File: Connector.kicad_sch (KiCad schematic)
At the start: 6 parts, among them J1 UJ20-C-H-G-SMT-1-P16-TR, J2 Conn_01x02_Socket, J3 DF40C, J4 DF40C

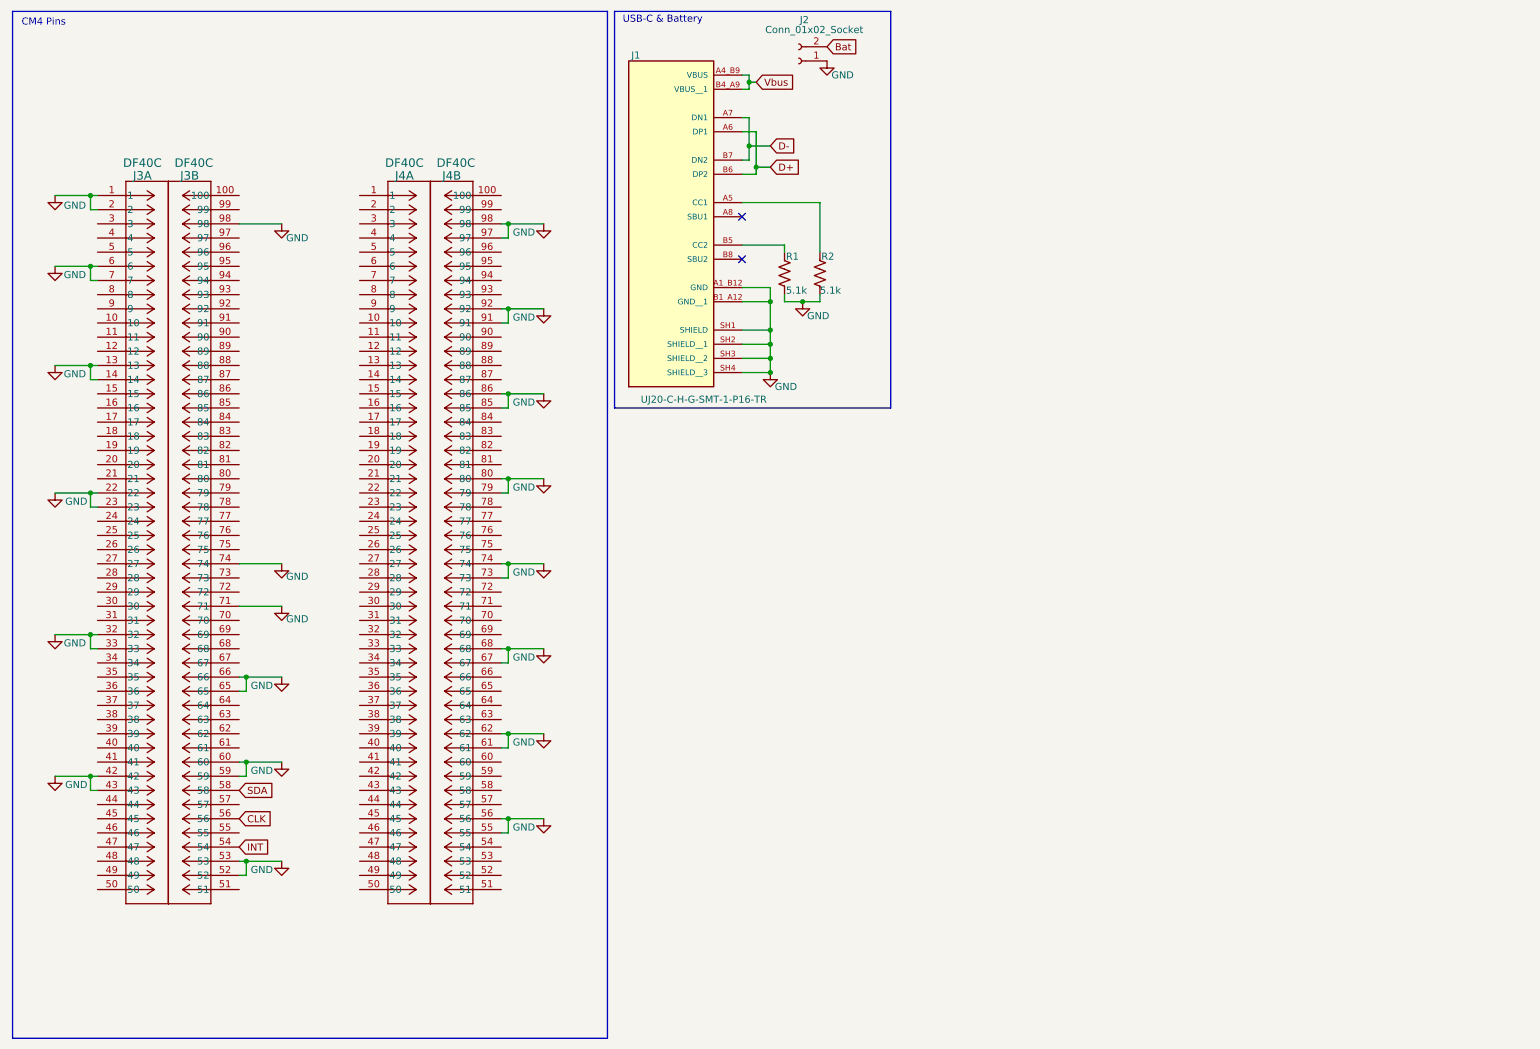
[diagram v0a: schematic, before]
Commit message: Final Schematic
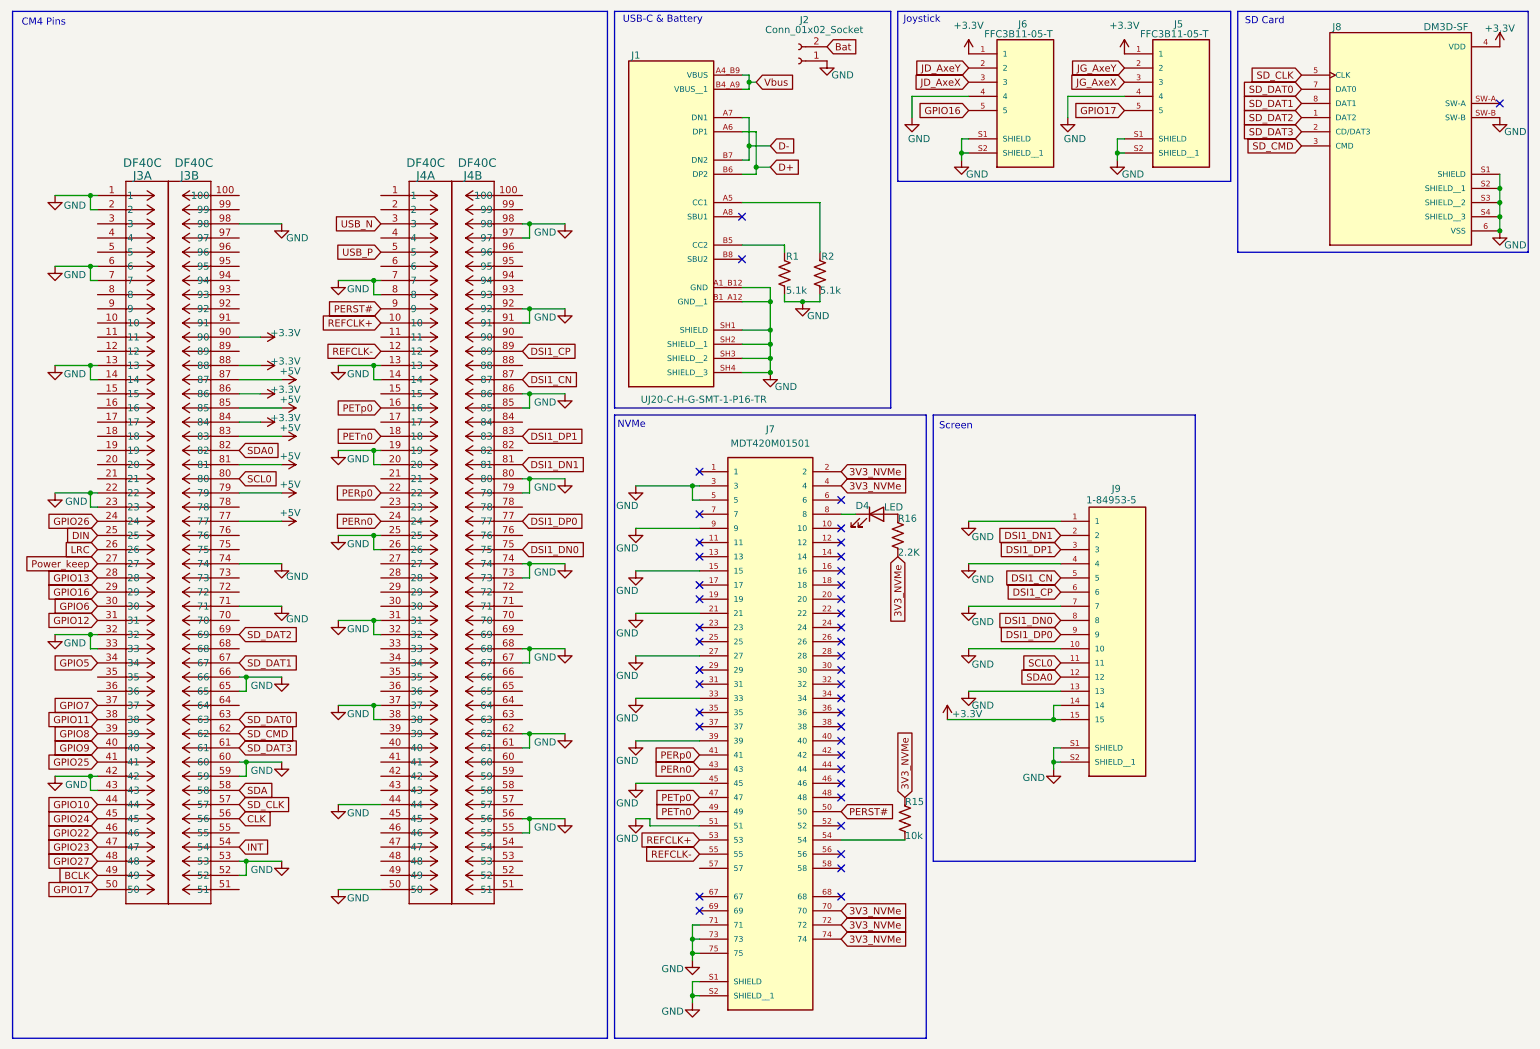
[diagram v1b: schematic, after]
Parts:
- added D4: LED, symbol Device:LED
- added J5, J6: FFC3B11-05-T, FFC3B11-05-T:GCT_FFC3B11-05-T, symbol FFC3B11-05-T:FFC3B11-05-T
- added J7: MDT420M01501, MDT420M01501:AMPHENOL_MDT420M01501, symbol MDT420M01501:MDT420M01501
- added J8: DM3D-SF, DM3D-SF:HRS_DM3D-SF, symbol DM3D-SF:DM3D-SF
- added J9: 1-84953-5, 1-84953-5:TE_1-84953-5, symbol Conn_FPC_15p:1-84953-5
- added R15: 10k, symbol Device:R_US
- added R16: 2.2K, symbol Device:R_US
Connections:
- net GND: now also J4.13, J4.14, J4.19, J4.20, J4.25, J4.26, J4.31, J4.32, J4.37, J4.38, J4.44, J4.50, J4.7, J4.8, J5.4, J5.S1 (SHIELD), J5.S2 (SHIELD__1), J6.4, J6.S1 (SHIELD), J6.S2 (SHIELD__1), J7.15, J7.21, J7.27, J7.3, J7.33, J7.39, J7.45, J7.5, J7.51, J7.71, J7.73, J7.75, J7.9, J7.S1 (SHIELD), J7.S2 (SHIELD__1), J8.6 (VSS), J8.S1 (SHIELD), J8.S2 (SHIELD__1), J8.S3 (SHIELD__2), J8.S4 (SHIELD__3), J8.SW-B, J9.1, J9.10, J9.13, J9.4, J9.7, J9.S1 (SHIELD), J9.S2 (SHIELD__1)
- net GPIO26: now reaches J3.24
- net DIN: now reaches J3.25
- net LRC: now reaches J3.26
- net Power_keep: now reaches J3.27
- net GPIO13: now reaches J3.28
- net GPIO16: now reaches J3.29
- net GPIO16: now also J6.5
- net GPIO6: now reaches J3.30
- net GPIO12: now reaches J3.31
- net GPIO5: now reaches J3.34
- net GPIO7: now reaches J3.37
- net GPIO11: now reaches J3.38
- net GPIO8: now reaches J3.39
- net GPIO9: now reaches J3.40
- net GPIO25: now reaches J3.41
- net GPIO10: now reaches J3.44
- net GPIO24: now reaches J3.45
- net GPIO22: now reaches J3.46
- net GPIO23: now reaches J3.47
- net GPIO27: now reaches J3.48
- net BCLK: now reaches J3.49
- net GPIO17: now reaches J3.50
- net GPIO17: now also J5.5
- net SD_CLK: now reaches J3.57
- net SD_CLK: now also J8.5 (CLK)
- net SD_DAT3: now reaches J3.61
- net SD_DAT3: now also J8.2 (CD/DAT3)
- net SD_CMD: now reaches J3.62
- net SD_CMD: now also J8.3 (CMD)
- net SD_DAT0: now reaches J3.63
- net SD_DAT0: now also J8.7 (DAT0)
- net SD_DAT1: now reaches J3.67
- net SD_DAT1: now also J8.8 (DAT1)
- net SD_DAT2: now reaches J3.69
- net SD_DAT2: now also J8.1 (DAT2)
- net +5V: now reaches J3.77
- net +5V: now also J3.79, J3.81, J3.83, J3.85, J3.87
- net SCL0: now reaches J3.80
- net SCL0: now also J9.11
- net SDA0: now reaches J3.82
- net SDA0: now also J9.12
- net +3.3V: now reaches J3.84
- net +3.3V: now also J3.86, J3.88, J3.90, J5.1, J6.1, J8.4 (VDD), J9.14, J9.15
- net REFCLK+: now reaches J4.10
- net REFCLK+: now also J7.53
- net REFCLK-: now reaches J4.12
- net REFCLK-: now also J7.55
- net PETp0: now reaches J4.16
- net PETp0: now also J7.47
- net PETn0: now reaches J4.18
- net PETn0: now also J7.49
- net PERp0: now reaches J4.22
- net PERp0: now also J7.41
- net PERn0: now reaches J4.24
- net PERn0: now also J7.43
- net USB_N: now reaches J4.3
- net USB_P: now reaches J4.5
- net PERST#: now reaches J4.9
- net PERST#: now also J7.50
- net DSI1_DN0: now reaches J4.75
- net DSI1_DN0: now also J9.8
- net DSI1_DP0: now reaches J4.77
- net DSI1_DP0: now also J9.9
- net DSI1_DN1: now reaches J4.81
- net DSI1_DN1: now also J9.2
- net DSI1_DP1: now reaches J4.83
- net DSI1_DP1: now also J9.3
- net DSI1_CN: now reaches J4.87
- net DSI1_CN: now also J9.5
- net DSI1_CP: now reaches J4.89
- net DSI1_CP: now also J9.6
- new net: D4.1 (K), J7.8
- new net: D4.2 (A), R16.1
- new net: J7.54, R15.2
- new net 3V3_NVMe: J7.2, J7.4, J7.70, J7.72, J7.74, R15.1, R16.2
- new net JD_AxeX: J6.3
- new net JD_AxeY: J6.2
- new net JG_AxeX: J5.3
- new net JG_AxeY: J5.2
- no-connect marks 2 -> 42
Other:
- note added: "Joystick"
- note added: "NVMe"
- note added: "SD Card"
- note added: "Screen"
- moved on the sheet: J4A, J4B
